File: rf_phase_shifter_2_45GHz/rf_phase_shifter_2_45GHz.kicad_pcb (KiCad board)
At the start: 2 copper layers, 12 parts, among them J1 Conn_Coaxial, J2 Conn_Coaxial, J3 Conn_Coaxial

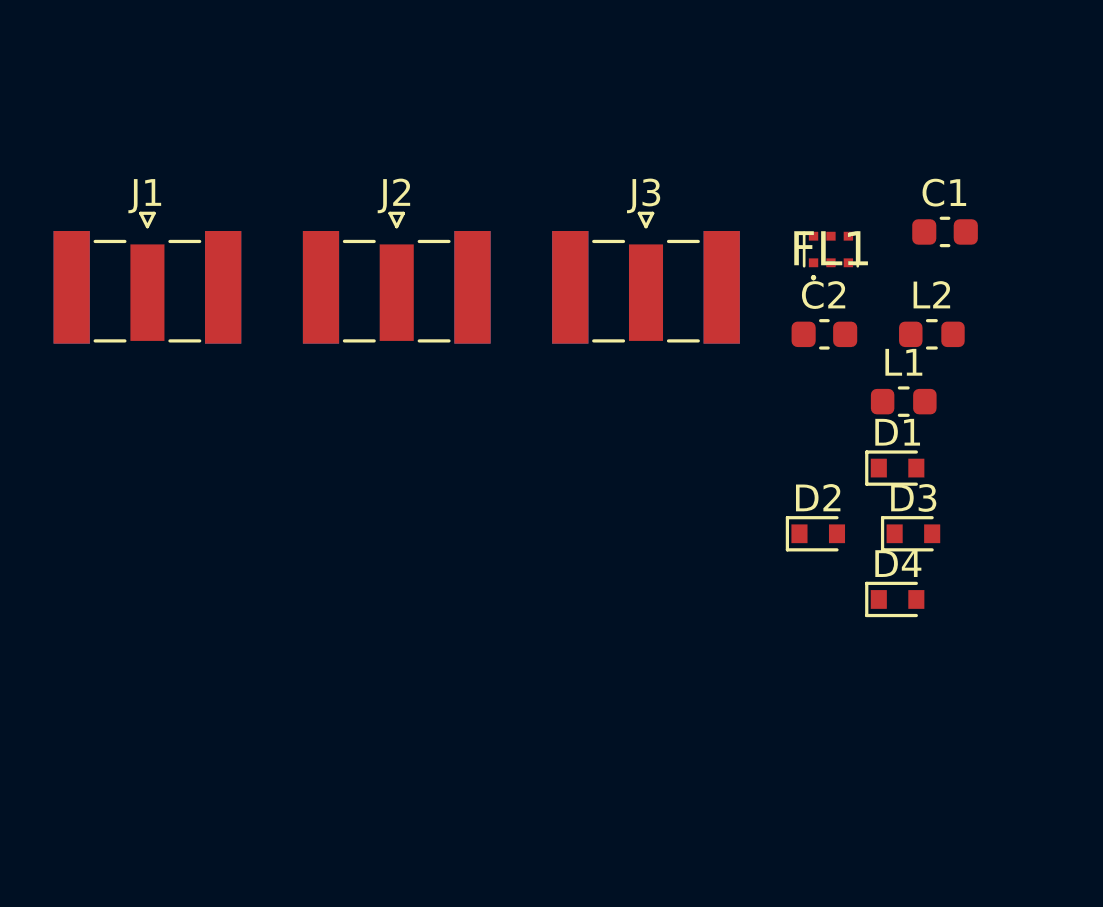
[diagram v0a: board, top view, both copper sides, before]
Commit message: Update rf_phase_shifter_2_45GHz.kicad_pcb
update
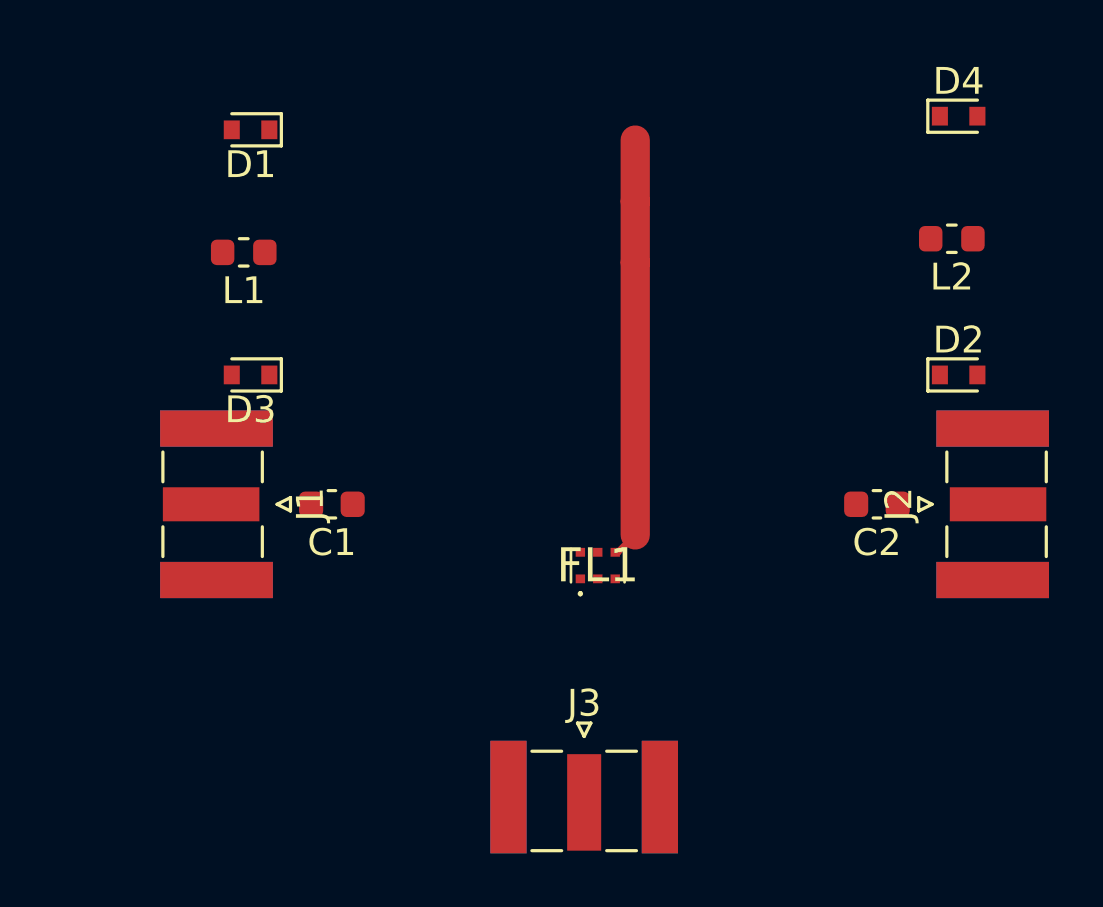
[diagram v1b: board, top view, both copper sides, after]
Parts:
- moved D1 27.2 mm to (90.9, 78.7), turned to 180 degrees
- moved D3 25.4 mm to (90.9, 87.9), turned to 180 degrees
- moved L1 25.2 mm to (90.7, 83.3), turned to 180 degrees
- moved C1 25.0 mm to (94.0, 92.7), turned to 180 degrees
- moved J2 23.7 mm to (118.6, 92.7), turned to 90 degrees
- moved J3 19.2 mm to (103.4, 103.6)
- moved D4 18.2 mm to (117.3, 78.2)
- moved FL1 14.7 mm to (103.9, 95.0)
- moved J1 8.50 mm to (89.7, 92.7), turned to 270 degrees
- moved D2 7.91 mm to (117.3, 87.9)
- moved C2 6.64 mm to (114.3, 92.7), turned to 180 degrees
- moved L2 3.64 mm to (117.1, 82.8), turned to 180 degrees
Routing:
- net Net-(D2-Pad1): track 0.00 -> 15.9 mm
